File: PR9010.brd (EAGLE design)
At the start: 71.6 x 80 mm, 60 parts, among them J1 M3_SCREW_POST, J2 AVR_SPI_PRG_6NS, SW1 SPST_TACT-KMR2, U1 SI4703, U2 TPA2005D1DGN, U3 Tiny85-20-SMT, Y1 32.768kHz

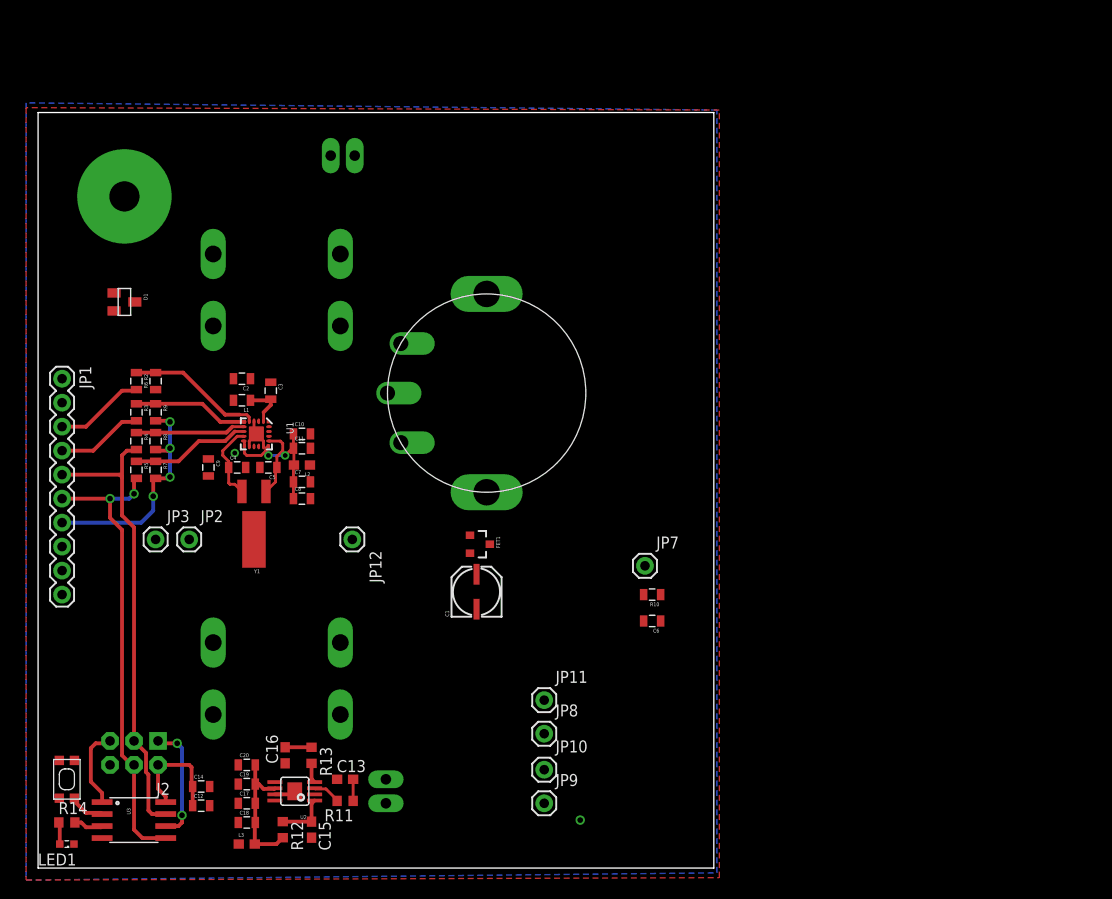
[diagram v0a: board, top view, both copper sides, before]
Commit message: Updated Sch & Layout
Began layout on the test board
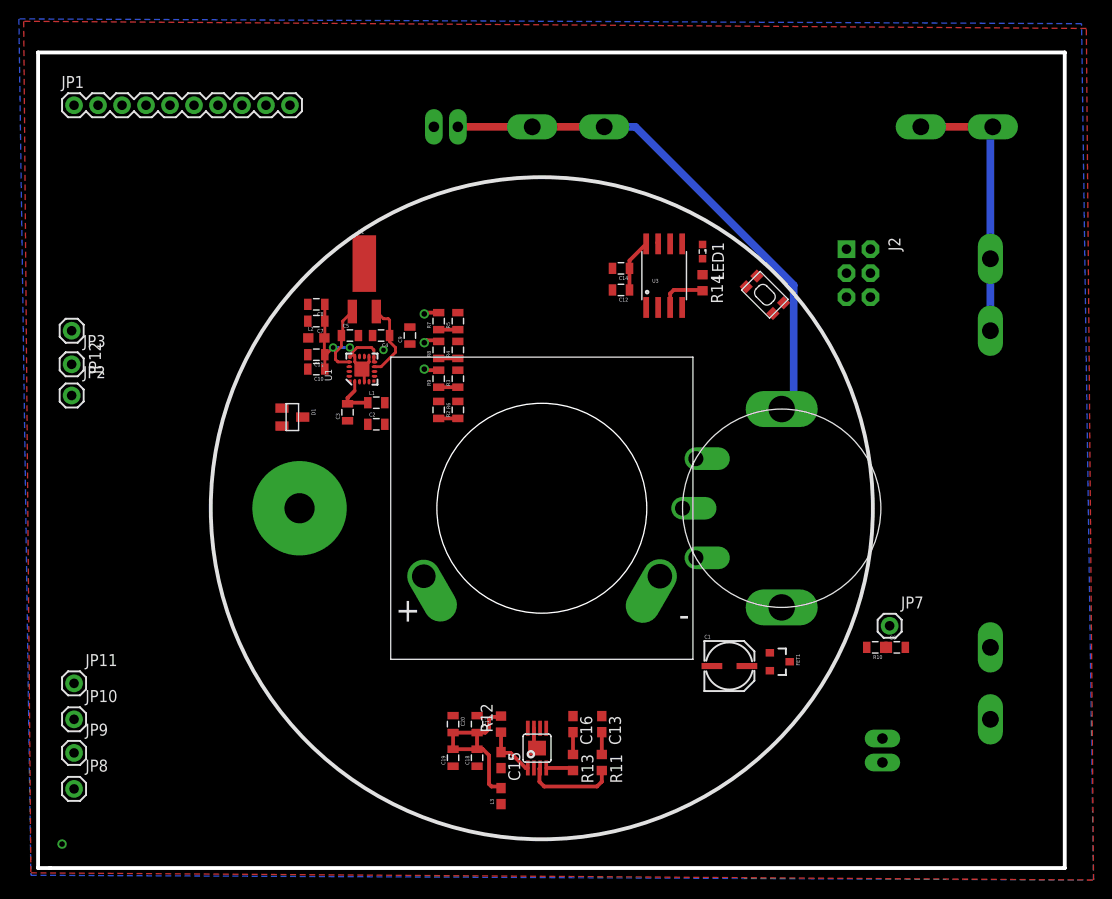
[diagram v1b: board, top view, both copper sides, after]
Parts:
- added U$3: CE32A_DAYTON_SPKR, PR_Libraries:CE32A_DAYTON_SPKR
- moved LED1 92.0 mm to (70.4, 65.3), turned to 270 degrees
- moved J2 92.0 mm to (86.9, 63.0), turned to 270 degrees
- moved SW1 90.0 mm to (77.0, 60.7), turned to 135 degrees
- moved R14 88.3 mm to (70.4, 62.0), turned to 270 degrees
- moved JP6 82.3 mm to (100.8, 40.1), turned to 90 degrees
- moved U3 80.5 mm to (66.3, 62.7), turned to 0 degrees
- moved C14 70.6 mm to (61.7, 63.5), turned to 180 degrees
- moved C12 70.4 mm to (61.7, 61.2), turned to 180 degrees
- moved JP5 58.6 mm to (76.7, 78.5), turned to 0 degrees
- moved JP13 52.8 mm to (89.4, 13.7)
- moved JP8 50.1 mm to (3.81, 8.38)
- moved JP10 50.1 mm to (3.81, 15.7)
- moved JP9 50.1 mm to (3.81, 12.2)
- moved JP11 49.8 mm to (3.81, 19.6)
- moved J1 37.9 mm to (27.7, 38.1)
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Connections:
- net OUT+: now also U$3.-
- net OUT-: now also U$3.+
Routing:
- net N$15: track 0.00 -> 56.2 mm
- net SDIO: track 49.5 -> 0.00 mm, vias 2 -> 0
- net SCLK: track 49.0 -> 0.18 mm
- net N$13: track 0.00 -> 31.3 mm
- net 3.3V: track 24.4 -> 4.83 mm, vias 4 -> 3
- net PB1: track 12.6 -> 0.00 mm, vias 2 -> 0
- net !RST-L: track 14.3 -> 2.03 mm
- net SDIO-L: track 12.7 -> 2.03 mm
- net !SEN-L: track 12.2 -> 2.03 mm
- net SCLK-L: track 11.6 -> 2.03 mm
- net !RST: track 9.50 -> 0.00 mm
- net !SEN: track 9.18 -> 0.00 mm
- net PB5: track 8.56 -> 0.00 mm
- net N$4: track 2.99 -> 9.69 mm
- net VCC: track 12.0 -> 5.61 mm
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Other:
- board size 71.6 x 80 mm -> 108.7 x 86.4 mm
